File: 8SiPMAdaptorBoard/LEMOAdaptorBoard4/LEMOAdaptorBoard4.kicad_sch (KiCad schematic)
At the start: 22 parts

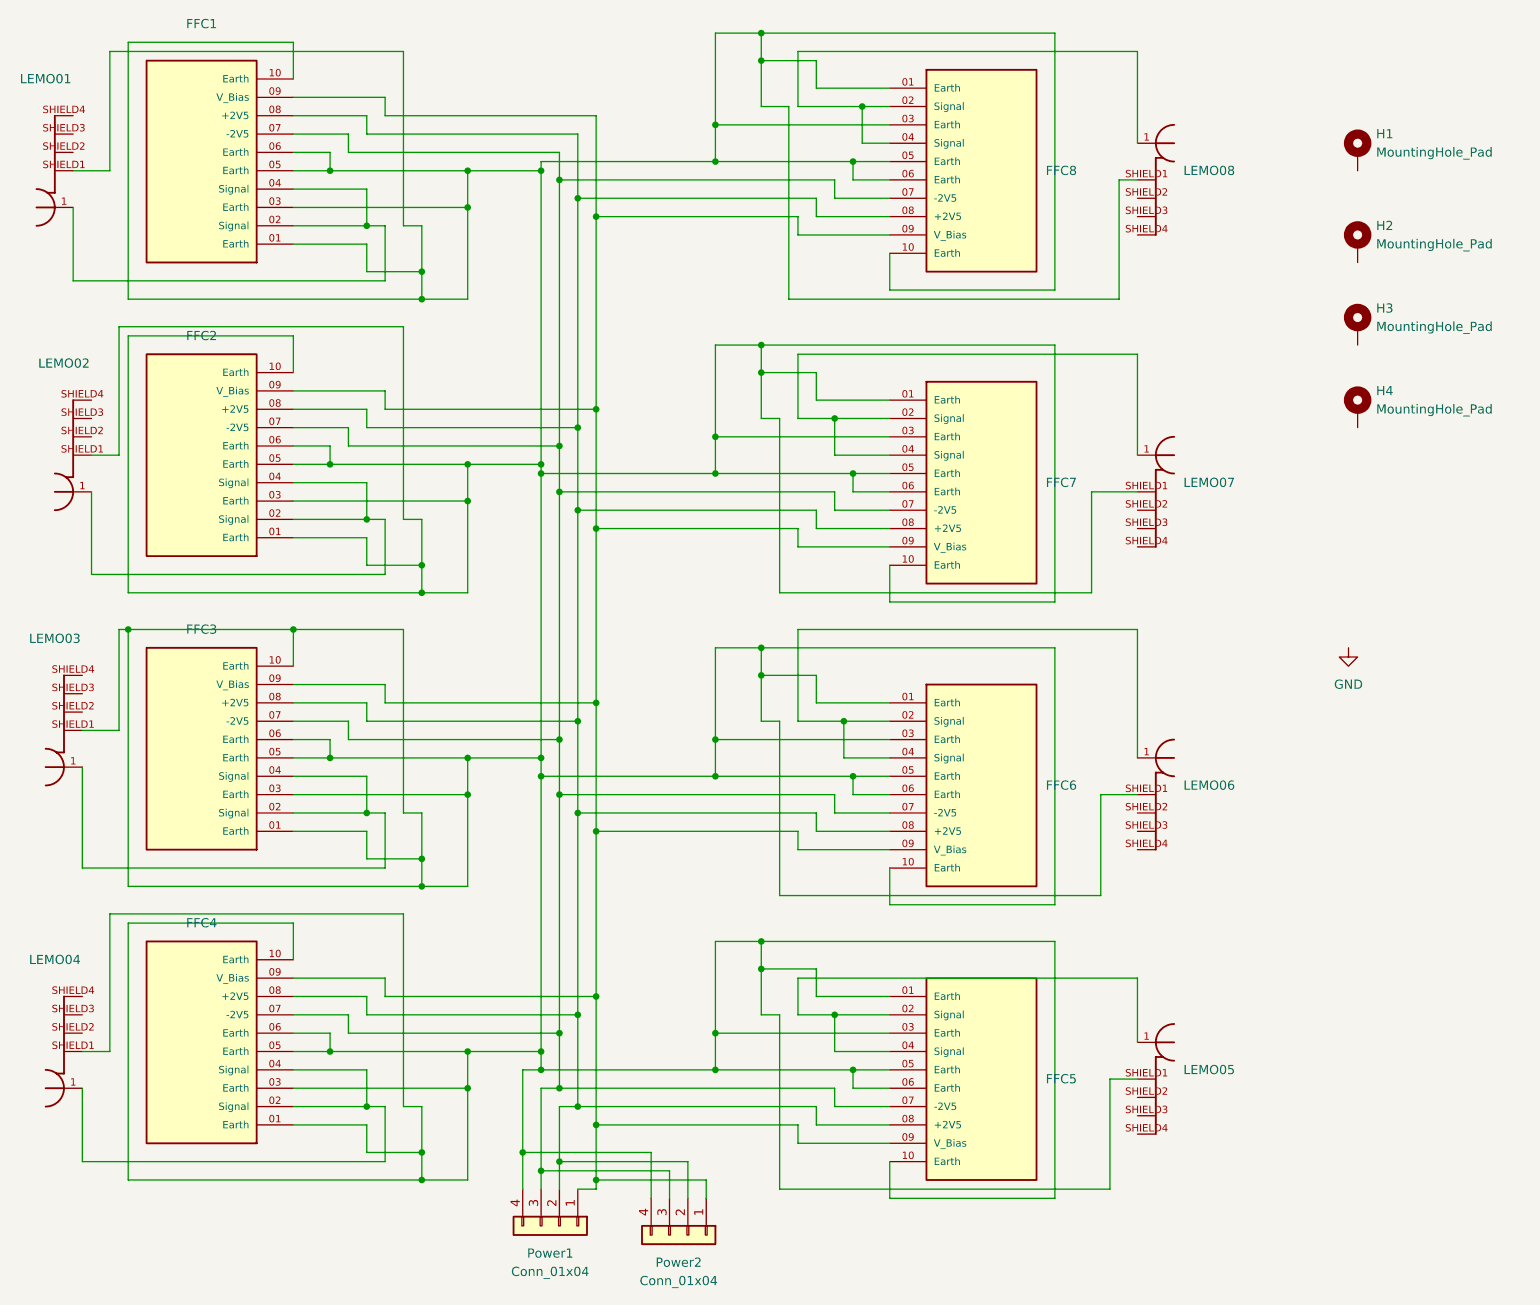
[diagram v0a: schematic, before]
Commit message: More update
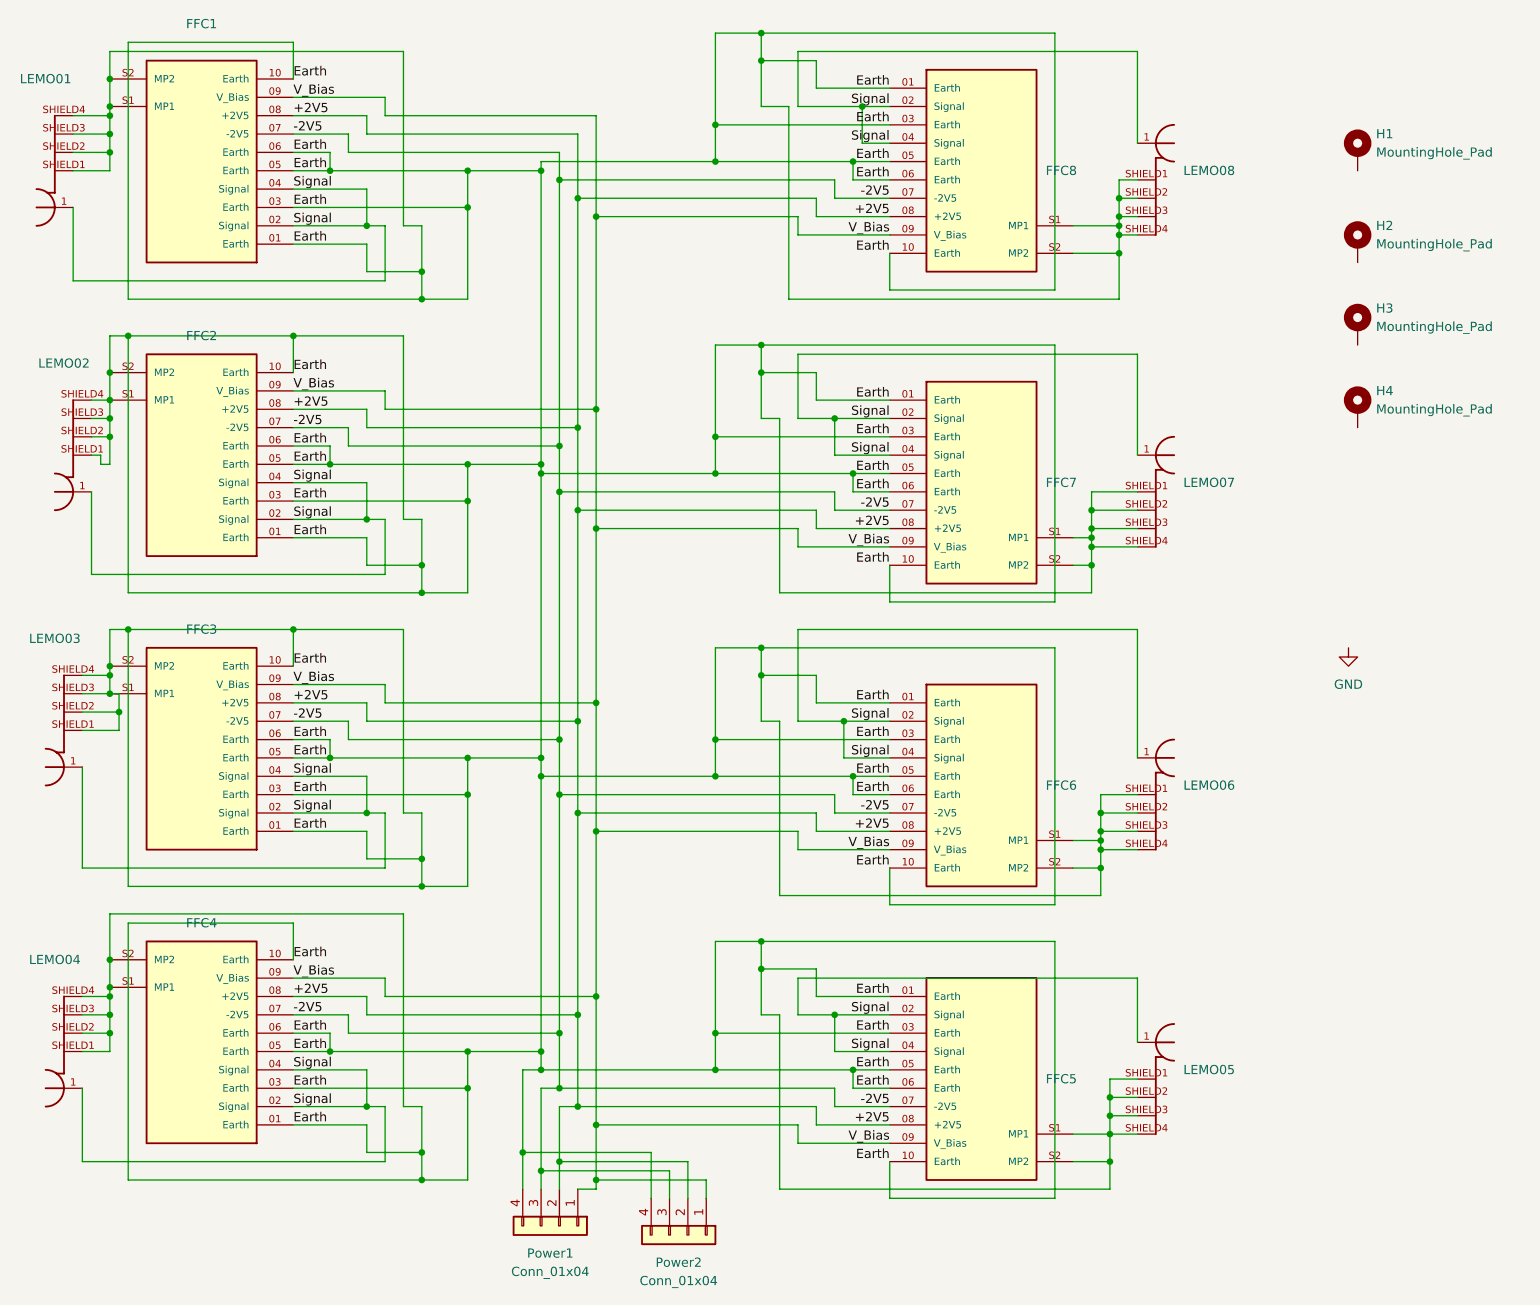
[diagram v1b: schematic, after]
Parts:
- Power1, Power2: footprint Connector:FanPinHeader_1x04_P2.54mm_Vertical -> Connector_PinHeader_2.54mm:PinHeader_1x04_P2.54mm_Horizontal
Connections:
- net Earth: now reaches FFC1.01 (Earth), FFC1.03 (Earth), FFC1.05 (Earth), FFC1.06 (Earth), FFC1.10 (Earth), FFC2.01 (Earth), FFC2.03 (Earth), FFC2.05 (Earth), FFC2.06 (Earth), FFC2.10 (Earth), FFC3.01 (Earth), FFC3.03 (Earth), FFC3.05 (Earth), FFC3.06 (Earth), FFC3.10 (Earth), FFC4.01 (Earth), FFC4.03 (Earth), FFC4.05 (Earth), FFC4.06 (Earth), FFC4.10 (Earth), FFC5.01 (Earth), FFC5.03 (Earth), FFC5.05 (Earth), FFC5.06 (Earth), FFC5.10 (Earth), FFC6.01 (Earth), FFC6.03 (Earth), FFC6.05 (Earth), FFC6.06 (Earth), FFC6.10 (Earth), FFC7.01 (Earth), FFC7.03 (Earth), FFC7.05 (Earth), FFC7.06 (Earth), FFC7.10 (Earth), FFC8.01 (Earth), FFC8.03 (Earth), FFC8.05 (Earth), FFC8.06 (Earth), FFC8.10 (Earth), LEMO01.SHIELD1, LEMO02.SHIELD1, LEMO03.SHIELD1, LEMO04.SHIELD1, LEMO05.SHIELD1, LEMO06.SHIELD1, LEMO07.SHIELD1, LEMO08.SHIELD1, Power1.4 (Pin_4), Power2.4 (Pin_4)
- net Earth: now also FFC1.S1 (MP1), FFC1.S2 (MP2), FFC2.S1 (MP1), FFC2.S2 (MP2), FFC3.S1 (MP1), FFC3.S2 (MP2), FFC4.S1 (MP1), FFC4.S2 (MP2), FFC5.S1 (MP1), FFC5.S2 (MP2), FFC6.S1 (MP1), FFC6.S2 (MP2), FFC7.S1 (MP1), FFC7.S2 (MP2), FFC8.S1 (MP1), FFC8.S2 (MP2), LEMO01.SHIELD2, LEMO01.SHIELD3, LEMO01.SHIELD4, LEMO02.SHIELD2, LEMO02.SHIELD3, LEMO02.SHIELD4, LEMO03.SHIELD2, LEMO03.SHIELD3, LEMO03.SHIELD4, LEMO04.SHIELD2, LEMO04.SHIELD3, LEMO04.SHIELD4, LEMO05.SHIELD2, LEMO05.SHIELD3, LEMO05.SHIELD4, LEMO06.SHIELD2, LEMO06.SHIELD3, LEMO06.SHIELD4, LEMO07.SHIELD2, LEMO07.SHIELD3, LEMO07.SHIELD4, LEMO08.SHIELD2, LEMO08.SHIELD3, LEMO08.SHIELD4
- net Signal: now reaches FFC2.02 (Signal), FFC2.04 (Signal), LEMO02.1
- net Signal: now also FFC1.02 (Signal), FFC1.04 (Signal), FFC3.02 (Signal), FFC3.04 (Signal), FFC4.02 (Signal), FFC4.04 (Signal), FFC5.02 (Signal), FFC5.04 (Signal), FFC6.02 (Signal), FFC6.04 (Signal), FFC7.02 (Signal), FFC7.04 (Signal), FFC8.02 (Signal), FFC8.04 (Signal), LEMO01.1, LEMO03.1, LEMO04.1, LEMO05.1, LEMO06.1, LEMO07.1, LEMO08.1
- net -2V5: now reaches FFC1.07 (-2V5), FFC2.07 (-2V5), FFC3.07 (-2V5), FFC4.07 (-2V5), FFC5.07 (-2V5), FFC6.07 (-2V5), FFC7.07 (-2V5), FFC8.07 (-2V5), Power1.3 (Pin_3), Power2.3 (Pin_3)
- net +2V5: now reaches FFC1.08 (+2V5), FFC2.08 (+2V5), FFC3.08 (+2V5), FFC4.08 (+2V5), FFC5.08 (+2V5), FFC6.08 (+2V5), FFC7.08 (+2V5), FFC8.08 (+2V5), Power1.2 (Pin_2), Power2.2 (Pin_2)
- net V_Bias: now reaches FFC1.09 (V_Bias), FFC2.09 (V_Bias), FFC3.09 (V_Bias), FFC4.09 (V_Bias), FFC5.09 (V_Bias), FFC6.09 (V_Bias), FFC7.09 (V_Bias), FFC8.09 (V_Bias), Power1.1 (Pin_1), Power2.1 (Pin_1)
